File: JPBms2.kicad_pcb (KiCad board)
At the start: 4 copper layers, 69 x 39 mm, 89 parts, among them J1 Conn_ARM_SWD_TagConnect_TC2030, J2 Barrel_Jack_MountingPin, Q1 AO3401A, Q10 AO3401A, Q11 2N7002, Q2 AO3401A, Q3 AO3400A, Q4 AO3400A, Q5 AO3401A, Q6 2N7002, Q7 2N7002, Q8 AO3401A, U1 ST715M25R, U2 STM32L053R8Tx, U3 ZXCT1107, U4 IRS2003, U5 IRS2003

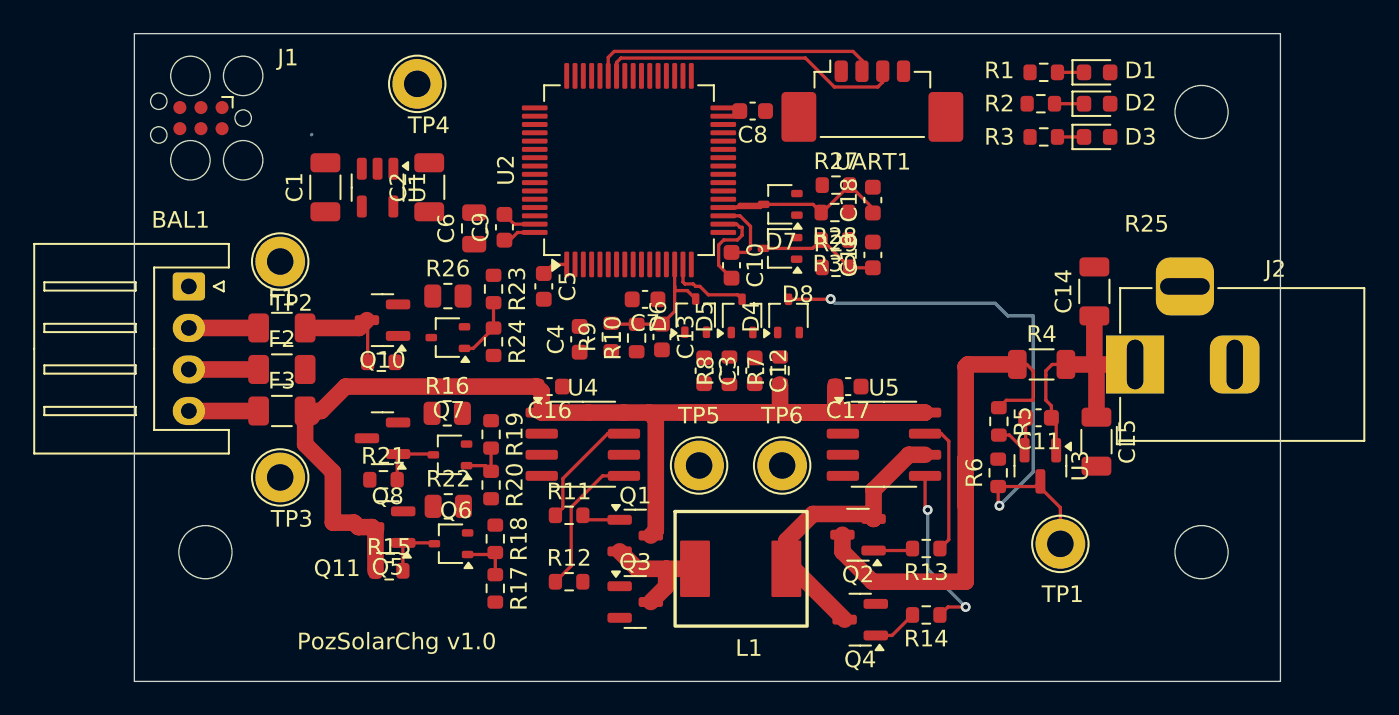
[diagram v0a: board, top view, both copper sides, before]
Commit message: Layout done
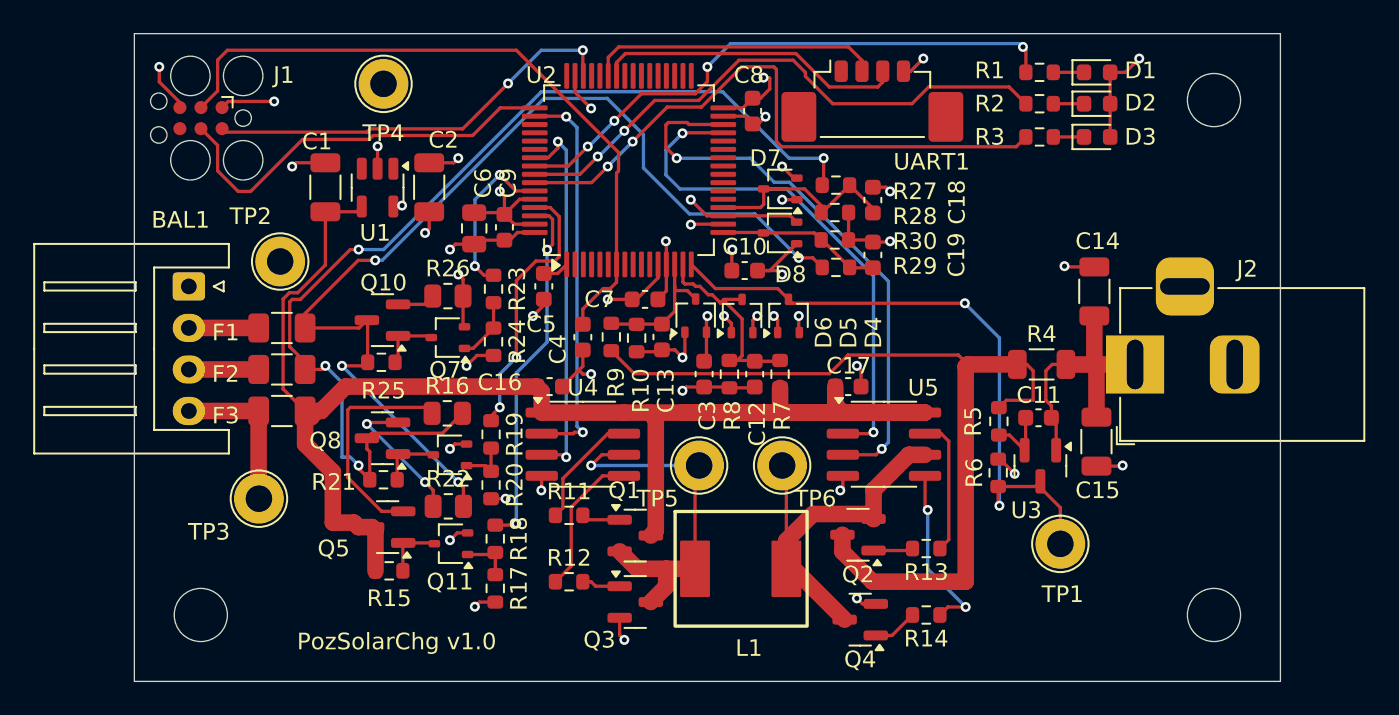
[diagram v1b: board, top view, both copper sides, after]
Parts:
- moved H3 3.85 mm to (161.0, 97.0)
- moved H2 3.79 mm to (100.0, 97.0)
- moved TP4 2.03 mm to (111.0, 65.0)
- moved TP3 1.81 mm to (103.5, 90.0)
- moved H1 1.04 mm to (161.0, 66.0)
- moved D7 0.93 mm to (134.9, 71.3)
- moved D8 0.93 mm to (134.9, 74.0)
- moved C10 0.85 mm to (132.7, 76.3), turned to 0 degrees
- moved R1 0.25 mm to (150.5, 64.3)
- moved R3 0.25 mm to (150.5, 68.2)
- moved C4 0.23 mm to (123.0, 80.3), turned to -90 degrees
- moved C12 0.20 mm to (133.3, 82.5)
- moved C3 0.20 mm to (130.3, 82.5)
- moved R7 0.20 mm to (134.9, 82.5)
- moved R8 0.20 mm to (131.8, 82.5)
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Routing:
- net GND: track 7.73 -> 76.5 mm, vias 0 -> 34
- net CELL_8V: track 0.00 -> 63.7 mm, vias 0 -> 4
- net CELL_4V: track 6.47 -> 62.4 mm, vias 0 -> 4
- net /MCU/NRST: track 0.00 -> 41.7 mm
- net /MCU/LED_ERROR: track 0.00 -> 37.2 mm, vias 0 -> 2
- net /MCU/LED_ON: track 0.00 -> 34.6 mm, vias 0 -> 4
- net /MCU/LED_ACTIVE: track 0.00 -> 34.5 mm, vias 0 -> 2
- net DD_BOT_B: track 0.00 -> 34.4 mm, vias 0 -> 2
- net VDD: track 6.49 -> 40.1 mm, vias 0 -> 13
- net DD_TOP_B: track 0.00 -> 31.7 mm, vias 0 -> 2
- net /MCU/SWDIO: track 0.00 -> 25.4 mm, vias 0 -> 2
- net /MCU/SWCLK: track 0.02 -> 24.6 mm
- net DD_TOP_A: track 0.00 -> 23.8 mm, vias 0 -> 2
- net DD_BOT_A: track 0.00 -> 22.8 mm, vias 0 -> 2
- net NBAL_3: track 0.00 -> 21.7 mm, vias 0 -> 2
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- added copper zone on In1.Cu, net GND
- added copper zone on In2.Cu, net VDD
